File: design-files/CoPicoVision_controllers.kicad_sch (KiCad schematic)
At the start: 34 parts, among them J401 Controller 1, J402 Controller 2, Q401 2N3904, Q402 2N3904, U103 74ACT05, U401 74LS541, U402 74LS541, U403 74HCT00

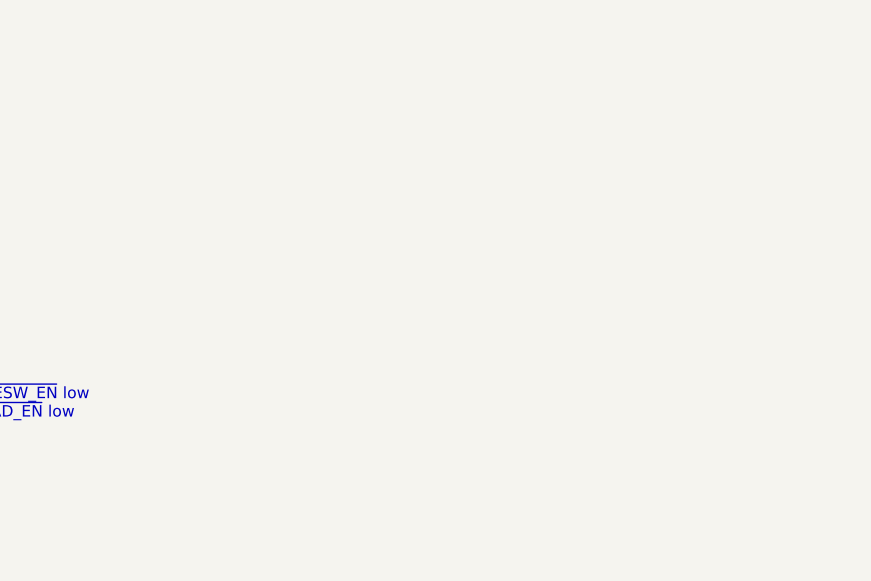
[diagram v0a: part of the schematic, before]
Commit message: Final controller checkpoint.  Managed to sqeeeze it all onto the board.
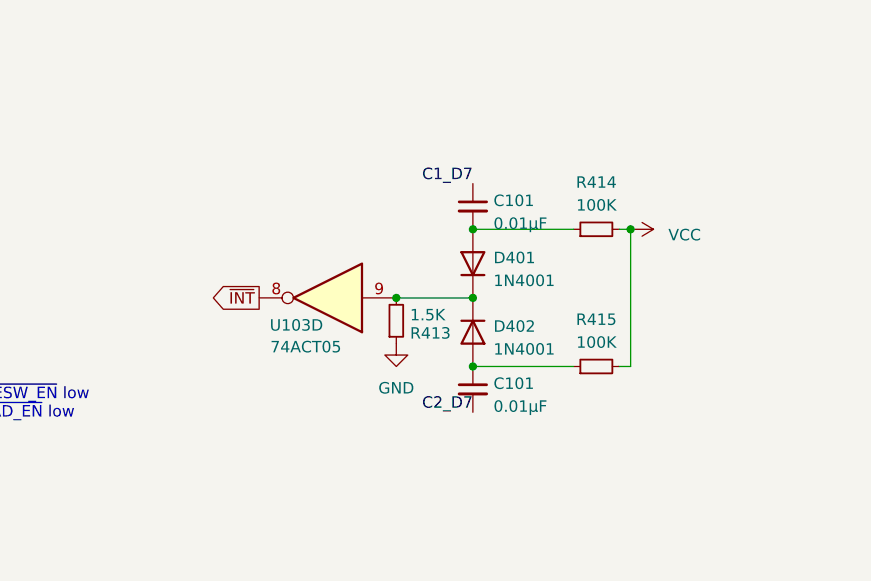
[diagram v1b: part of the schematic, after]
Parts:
- added C101 (x2): 0.01µF, Capacitor_THT:C_Disc_D3.8mm_W2.6mm_P2.50mm, symbol Device:C_Small
- added D401, D402: 1N4001, Diode_THT:D_DO-41_SOD81_P10.16mm_Horizontal, symbol Diode:1N4001
- added R413: 1.5K, Resistor_THT:R_Axial_DIN0207_L6.3mm_D2.5mm_P7.62mm_Horizontal, symbol Device:R_Small
- added R414, R415: 100K, Resistor_THT:R_Axial_DIN0207_L6.3mm_D2.5mm_P7.62mm_Horizontal, symbol Device:R_Small
- added unit 4 of U103
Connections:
- net C1_D7: now also C101.1
- net C2_D7: now also C101.2
- net GND: now also R413.1
- net VCC: now also R414.2, R415.2
- new net: C101.1, D402.2 (A), R415.1
- new net: D401.1 (K), D402.1 (K), R413.2, U103.9
- new net: C101.2, D401.2 (A), R414.1
- new net ~{INT}: U103.8
